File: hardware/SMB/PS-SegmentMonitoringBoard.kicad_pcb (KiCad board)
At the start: 4 copper layers, 86.5 x 85 mm, 126 parts, among them IC1 BQ79616PAPR, J1 voltTapConn, J2 highSideConn, J3 lowSideConn, J4 thermsConn, Q1 ZXTN4004KTC

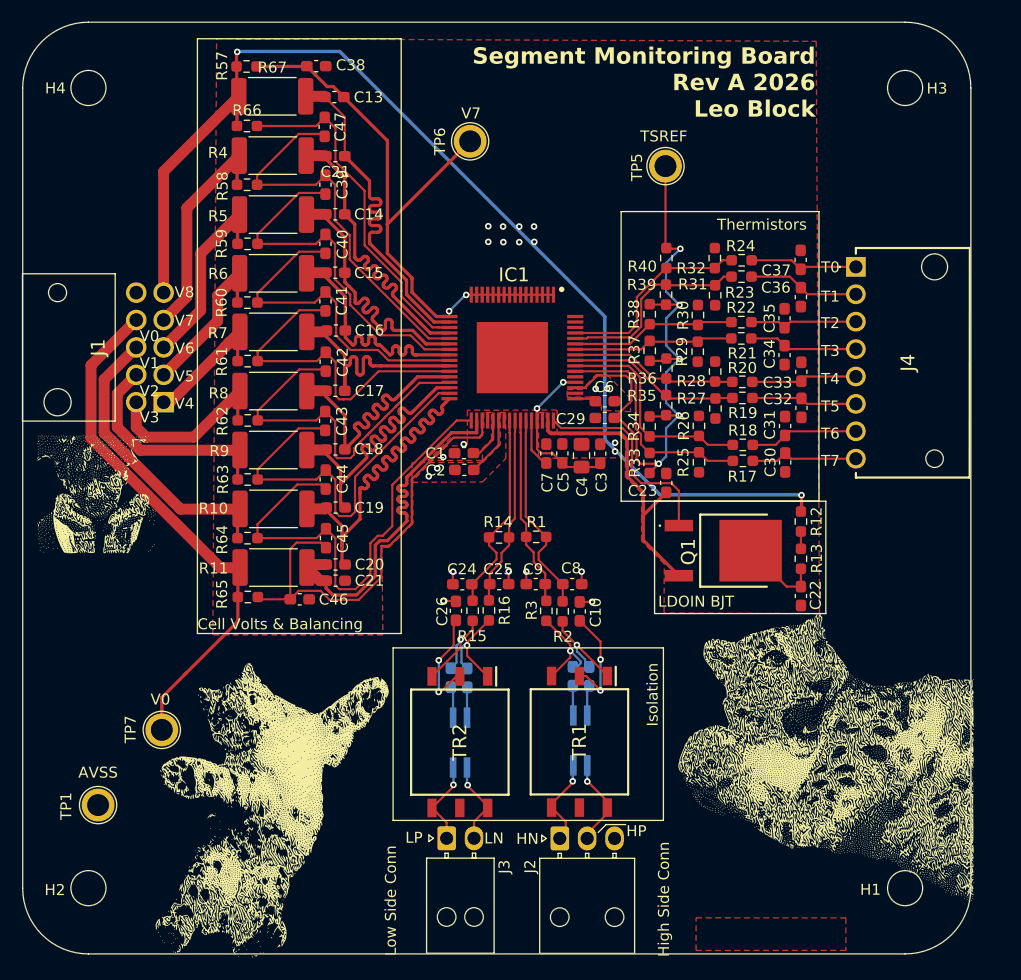
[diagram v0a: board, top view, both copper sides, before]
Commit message: added ntcs gnda
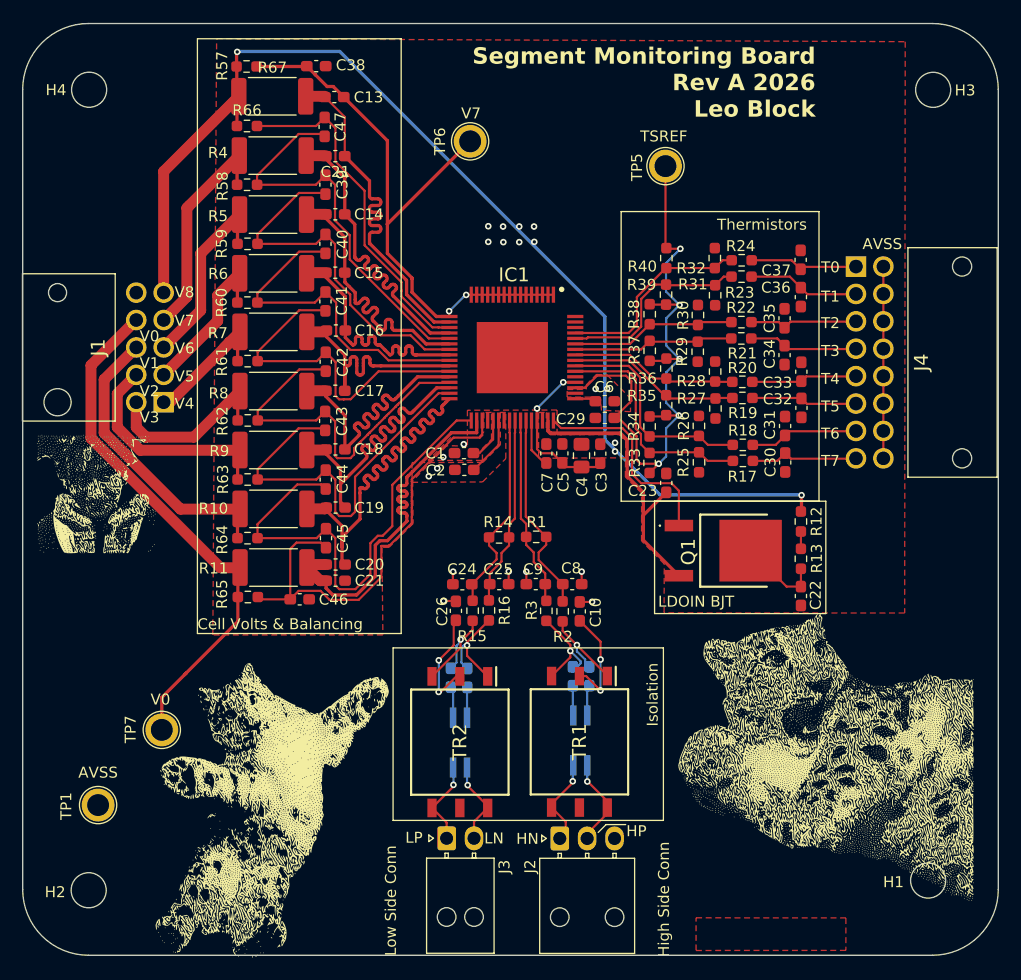
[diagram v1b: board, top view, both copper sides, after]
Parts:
- J4: value thermsConn -> thermConn; footprint LHRS_Connectors:Molex_Nano-Fit_105313-xx08_1x08_P2.50mm_Horizontal -> Custom-Footprints:1053141116
- moved H3 2.57 mm to (155.9, 64.1)
- moved H1 2.21 mm to (155.4, 136.2)
- moved H2 0.19 mm to (78.8, 137.1)
- moved H4 0.17 mm to (78.9, 64.1)
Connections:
- J4 pad 1: /Thermistors/TEMP_0 -> /Thermistors/TEMP_7
- J4 pad 2: /Thermistors/TEMP_1 -> /Thermistors/TEMP_6
- J4 pad 3: /Thermistors/TEMP_2 -> /Thermistors/TEMP_5
- J4 pad 4: /Thermistors/TEMP_3 -> /Thermistors/TEMP_4
- J4 pad 5: /Thermistors/TEMP_4 -> /Thermistors/TEMP_3
- J4 pad 6: /Thermistors/TEMP_5 -> /Thermistors/TEMP_2
- J4 pad 7: /Thermistors/TEMP_6 -> /Thermistors/TEMP_1
- J4 pad 8: /Thermistors/TEMP_7 -> /Thermistors/TEMP_0
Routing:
- net AVSS: track 6.87 -> 24.4 mm
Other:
- board size 86.5 x 85 mm -> 89 x 85 mm
